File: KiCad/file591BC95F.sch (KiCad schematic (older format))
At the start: 54 parts, among them J203 V4, P201 Power Pole, P203 Power Pole, Q201 MUN5213DW1, Q202 DMP4025LSD, Q203 RJK0354DSP, U201 DAC081C085, U202 OPA171, U203 LTC3600, U204 MIC2196

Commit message: Design Updates
Defining parts and footprints
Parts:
- R214: Digi-Key Part No. 311-10.0KCRCT-ND -> 311-10KLGCT-ND; Link <a href=\"https://www.digikey.com/products/en?keywords=311-10.0KCRCT-ND\">Link</a> -> <a href=\"https://www.digikey.com/products/en?keywords=311-10KLGCT-ND\">Link</a>; Manufacturer PN RC0805FR-0710KL -> AC0805FR-0710KL
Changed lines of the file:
@@
 F 2 "Resistors_SMD:R_0805" V 2080 6200 50  0001 C CNN
 F 3 "" H 2150 6200 50  0000 C CNN
-F 4 "311-10.0KCRCT-ND" H 2150 6200 50  0001 C CNN "Digi-Key Part No."
-F 5 "<a href=\"https://www.digikey.com/products/en?keywords=311-10.0KCRCT-ND\">Link</a>" H 2150 6200 60  0001 C CNN "Link"
+F 4 "311-10KLGCT-ND" H 2150 6200 50  0001 C CNN "Digi-Key Part No."
+F 5 "<a href=\"https://www.digikey.com/products/en?keywords=311-10KLGCT-ND\">Link</a>" H 2150 6200 60  0001 C CNN "Link"
 F 6 "Yageo" H 2150 6200 50  0001 C CNN "Manufacturer"
-F 7 "RC0805FR-0710KL" H 2150 6200 50  0001 C CNN "Manufacturer PN"
+F 7 "AC0805FR-0710KL" H 2150 6200 50  0001 C CNN "Manufacturer PN"
 F 8 "RES SMD 10K OHM 1% 1/8W 0805" H 2150 6200 50  0001 C CNN "Description"
 	1    2150 6200

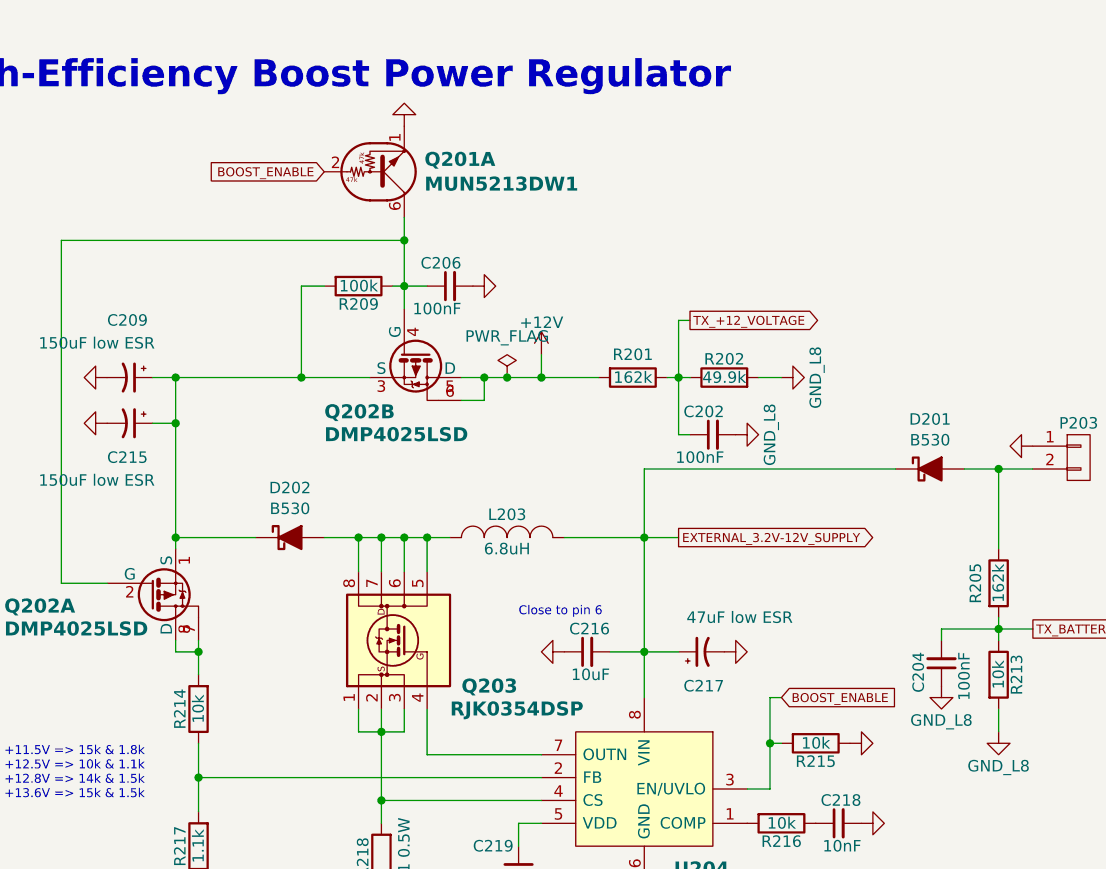
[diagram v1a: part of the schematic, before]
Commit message: Design Updates
Updating schematic parts
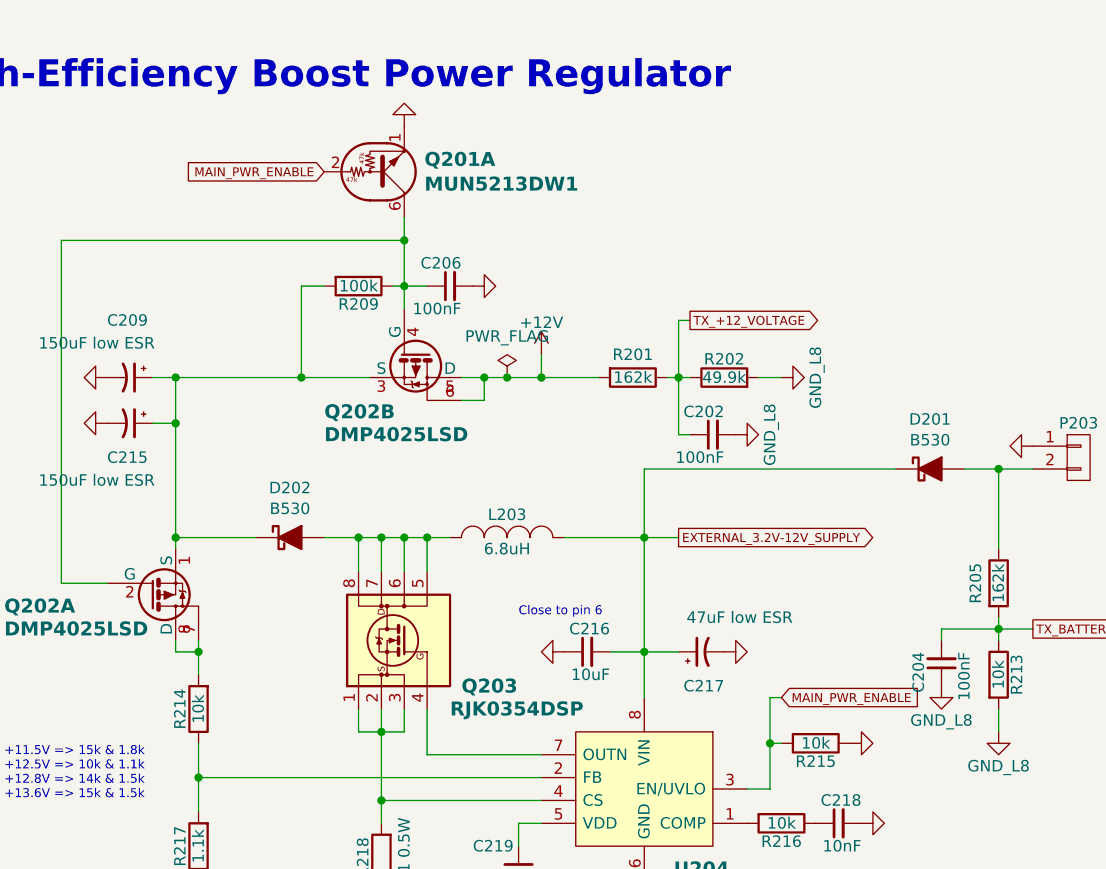
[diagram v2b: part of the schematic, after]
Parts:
- C209, C214, C215, C217: footprint Capacitors_SMD:C_2917_7343_Metric_HandSoldering -> Capacitors_SMD:C_2917
- R202: footprint Resistors_SMD:R_0805_HandSoldering -> Resistors_SMD:R_0805
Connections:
- net labels added: MAIN_PWR_ENABLE
- net labels removed: BOOST_ENABLE
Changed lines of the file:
@@
 F 0 "C214" H 8900 2850 50  0000 L CNN
 F 1 "47uF low ESR" H 9350 2850 50  0000 L CNN
-F 2 "Capacitors_SMD:C_2917_7343_Metric_HandSoldering" H 9200 2850 50  0001 C CNN
+F 2 "Capacitors_SMD:C_2917" H 9200 2850 50  0001 C CNN
 F 3 "" H 9200 2850 50  0001 C CNN
 F 4 "399-3904-1-ND" H 9200 2850 50  0001 C CNN "Digi-Key Part No."
@@
 F 0 "C215" V 2000 4850 50  0000 L CNN
 F 1 "150uF low ESR" V 2100 4550 50  0000 L CNN
-F 2 "Capacitors_SMD:C_2917_7343_Metric_HandSoldering" H 1850 4950 50  0001 C CNN
+F 2 "Capacitors_SMD:C_2917" H 1850 4950 50  0001 C CNN
 F 3 "" H 1850 4950 50  0001 C CNN
 F 4 "478-5253-1-ND" H 1850 4950 50  0001 C CNN "Digi-Key Part No."
@@
 F 0 "R202" V 4530 4750 50  0000 C CNN
 F 1 "49.9k" V 4450 4750 50  0000 C CNN
-F 2 "Resistors_SMD:R_0805_HandSoldering" V 4380 4750 50  0001 C CNN
+F 2 "Resistors_SMD:R_0805" V 4380 4750 50  0001 C CNN
 F 3 "" H 4450 4750 50  0001 C CNN
 F 4 "YAG4990CT-ND" H 4450 4750 50  0001 C CNN "Digi-Key Part No."
@@
 	4250 4500 4250 4750
 Text GLabel 4700 6150 2    39   Input ~ 0
-BOOST_ENABLE
+MAIN_PWR_ENABLE
 Wire Wire Line
 	4700 6150 4650 6150
@@
 +11.5V => 15k & 1.8k\n+12.5V => 10k & 1.1k\n+12.8V => 14k & 1.5k\n+13.6V => 15k & 1.5k
 Text GLabel 2700 3850 0    39   Input ~ 0
-BOOST_ENABLE
+MAIN_PWR_ENABLE
 $Comp
 L Device:D_Schottky_ALT D202
@@
 F 0 "C209" V 1600 4650 50  0000 L CNN
 F 1 "150uF low ESR" V 1700 4350 50  0000 L CNN
-F 2 "Capacitors_SMD:C_2917_7343_Metric_HandSoldering" H 1850 4750 50  0001 C CNN
+F 2 "Capacitors_SMD:C_2917" H 1850 4750 50  0001 C CNN
 F 3 "" H 1850 4750 50  0001 C CNN
 F 4 "478-5253-1-ND" H 1850 4750 50  0001 C CNN "Digi-Key Part No."
@@
 F 0 "C217" V 4200 5850 50  0000 L CNN
 F 1 "47uF low ESR" V 4500 5550 50  0000 L CNN
-F 2 "Capacitors_SMD:C_2917_7343_Metric_HandSoldering" H 4350 5950 50  0001 C CNN
+F 2 "Capacitors_SMD:C_2917" H 4350 5950 50  0001 C CNN
 F 3 "" H 4350 5950 50  0001 C CNN
 F 4 "399-3904-1-ND" H 4350 5950 50  0001 C CNN "Digi-Key Part No."

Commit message: Design Updates
Updated schematics parts descriptions
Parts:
- L201: symbol FlexFox80-rescue:INDUCTOR_SMALL-ARDF-2-Band-MiniTx-rescue -> Device:INDUCTOR_SMALL
- P201: footprint (none) -> Oddities:Dummy_Empty_2
- P203: footprint (none) -> Connect:PowerPole-ASMPP30-1x2
- U201: symbol FlexFox80-rescue:DAC081C085-ARDF-2-Band-MiniTx-rescue -> Analog_DAC:DAC081C085
- U202: symbol FlexFox80-rescue:OPA171-ARDF-2-Band-MiniTx-rescue -> Amplifier_Operational:OPA171
- U203: symbol FlexFox80-rescue:LTC3600-ARDF-2-Band-MiniTx-rescue -> Regulator_Switching:LTC3600
- W204: symbol FlexFox80-rescue:TEST_SCOPE-ARDF-2-Band-MiniTx-rescue -> special:TEST_SCOPE
- W205: symbol FlexFox80-rescue:TEST_SCOPE-ARDF-2-Band-MiniTx-rescue -> special:TEST_SCOPE; Manufacturer (none) -> np
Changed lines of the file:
@@
 $EndDescr
 $Comp
-L FlexFox80-rescue:LTC3600-ARDF-2-Band-MiniTx-rescue U203
+L Regulator_Switching:LTC3600 U203
 U 1 1 58B77FB4
 P 7550 2500
@@
 $EndComp
 $Comp
-L FlexFox80-rescue:DAC081C085-ARDF-2-Band-MiniTx-rescue U201
+L Analog_DAC:DAC081C085 U201
 U 1 1 58B84991
 P 3600 2250
@@
 High-Efficiency Variable Buck Power Regulator
 $Comp
-L FlexFox80-rescue:OPA171-ARDF-2-Band-MiniTx-rescue U202
+L Amplifier_Operational:OPA171 U202
 U 1 1 59D417D4
 P 6000 2200
+AR Path="/59D417D4" Ref="U202"  Part="1"
+AR Path="/591BC960/59D417D4" Ref="U202"  Part="1"
 F 0 "U202" H 6000 2450 61  0000 L CNB
 F 1 "OPA171" H 6000 2350 61  0000 L CNB
@@
 F 0 "P203" H 6000 5250 50  0000 C CNN
 F 1 "Power Pole" V 6150 5100 50  0001 C CNN
-F 2 "" H 6000 5100 50  0001 C CNN
+F 2 "Connect:PowerPole-ASMPP30-1x2" H 6000 5100 50  0001 C CNN
 F 3 "" H 6000 5100 50  0001 C CNN
 F 4 "2243-ASMPP30-1X2-RK-ND" H 6000 5100 50  0001 C CNN "Digi-Key Part No."
@@
 	3800 1350 3800 1400
 $Comp
-L FlexFox80-rescue:INDUCTOR_SMALL-ARDF-2-Band-MiniTx-rescue L201
+L Device:INDUCTOR_SMALL L201
 U 1 1 5BF17B46
 P 4350 1650
@@
 NoConn ~ 6500 5150
 $Comp
-L FlexFox80-rescue:TEST_SCOPE-ARDF-2-Band-MiniTx-rescue W204
+L special:TEST_SCOPE W204
 U 1 1 5C0F212A
 P 9400 1500
@@
 $EndComp
 $Comp
-L FlexFox80-rescue:TEST_SCOPE-ARDF-2-Band-MiniTx-rescue W205
+L special:TEST_SCOPE W205
 U 1 1 5F84AD75
 P 4800 2250
@@
 F 4 "np" H 4800 2250 50  0001 C CNN "Digi-Key Part No."
 F 5 "np" H 4800 2250 60  0001 C CNN "Link"
+F 6 "np" H 4800 2250 50  0001 C CNN "Manufacturer"
 	1    4800 2250
 	-1   0    0    1
@@
 F 0 "P201" H 6300 5250 50  0000 C CNN
 F 1 "Power Pole" V 6450 5100 50  0000 C CNN
-F 2 "" H 6300 5100 50  0001 C CNN
+F 2 "Oddities:Dummy_Empty_2" H 6300 5100 50  0001 C CNN
 F 3 "" H 6300 5100 50  0001 C CNN
 F 4 "2243-ASMPP30-1X2-RK-ND" H 6300 5100 50  0001 C CNN "Digi-Key Part No."
